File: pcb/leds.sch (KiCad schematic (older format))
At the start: 15 parts, among them J11 +5V, J12 DATA, J13 GND

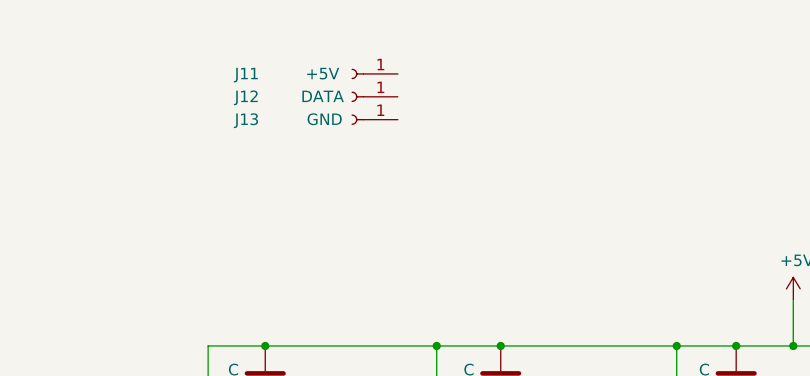
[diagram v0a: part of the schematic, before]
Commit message: update
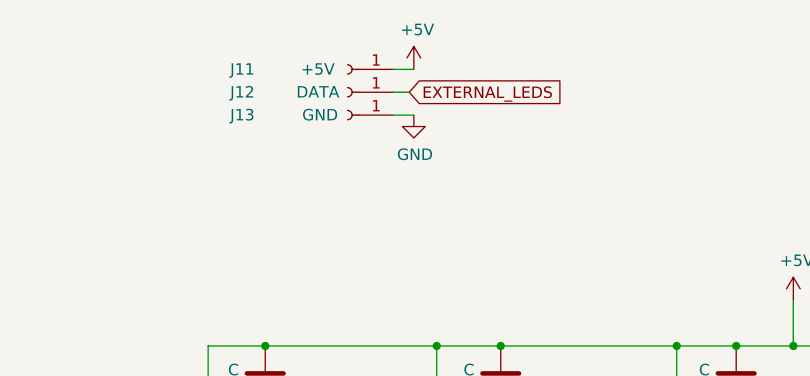
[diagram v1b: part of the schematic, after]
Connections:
- net labels added: EXTERNAL_LEDS
- wire segments 34 -> 37
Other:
- moved on the sheet: J11, J12, J13
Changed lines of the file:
@@
 L Connector:Conn_01x01_Female J?
 U 1 1 61EFE4C5
-P 4670 2340
+P 4650 2320
 AR Path="/61EFE4C5" Ref="J?"  Part="1"
 AR Path="/61B99CE8/61EFE4C5" Ref="J?"  Part="1"
 AR Path="/61B54BD1/61EFE4C5" Ref="J11"  Part="1"
-F 0 "J11" H 5130 2340 50  0000 C CNN
-F 1 "+5V" H 4800 2340 50  0000 C CNN
-F 2 "TestPoint:TestPoint_Pad_D2.0mm" H 4670 2340 50  0001 C CNN
-F 3 "~" H 4670 2340 50  0001 C CNN
-	1    4670 2340
+F 0 "J11" H 5110 2320 50  0000 C CNN
+F 1 "+5V" H 4780 2320 50  0000 C CNN
+F 2 "TestPoint:TestPoint_Pad_D2.0mm" H 4650 2320 50  0001 C CNN
+F 3 "~" H 4650 2320 50  0001 C CNN
+	1    4650 2320
 	-1   0    0    1
 $EndComp
@@
 L Connector:Conn_01x01_Female J?
 U 1 1 61EFE4CB
-P 4670 2440
+P 4650 2420
 AR Path="/61EFE4CB" Ref="J?"  Part="1"
 AR Path="/61B99CE8/61EFE4CB" Ref="J?"  Part="1"
 AR Path="/61B54BD1/61EFE4CB" Ref="J12"  Part="1"
-F 0 "J12" H 5130 2440 50  0000 C CNN
-F 1 "DATA" H 4800 2440 50  0000 C CNN
-F 2 "TestPoint:TestPoint_Pad_D2.0mm" H 4670 2440 50  0001 C CNN
-F 3 "~" H 4670 2440 50  0001 C CNN
-	1    4670 2440
+F 0 "J12" H 5110 2420 50  0000 C CNN
+F 1 "DATA" H 4780 2420 50  0000 C CNN
+F 2 "TestPoint:TestPoint_Pad_D2.0mm" H 4650 2420 50  0001 C CNN
+F 3 "~" H 4650 2420 50  0001 C CNN
+	1    4650 2420
 	-1   0    0    1
 $EndComp
@@
 L Connector:Conn_01x01_Female J?
 U 1 1 61EFE4D1
-P 4670 2540
+P 4650 2520
 AR Path="/61EFE4D1" Ref="J?"  Part="1"
 AR Path="/61B99CE8/61EFE4D1" Ref="J?"  Part="1"
 AR Path="/61B54BD1/61EFE4D1" Ref="J13"  Part="1"
-F 0 "J13" H 5130 2540 50  0000 C CNN
-F 1 "GND" H 4790 2540 50  0000 C CNN
-F 2 "TestPoint:TestPoint_Pad_D2.0mm" H 4670 2540 50  0001 C CNN
-F 3 "~" H 4670 2540 50  0001 C CNN
-	1    4670 2540
+F 0 "J13" H 5110 2520 50  0000 C CNN
+F 1 "GND" H 4770 2520 50  0000 C CNN
+F 2 "TestPoint:TestPoint_Pad_D2.0mm" H 4650 2520 50  0001 C CNN
+F 3 "~" H 4650 2520 50  0001 C CNN
+	1    4650 2520
 	-1   0    0    1
 $EndComp
+Text GLabel 4920 2420 2    50   Input ~ 0
+EXTERNAL_LEDS
+Wire Wire Line
+	4850 2420 4920 2420
+$Comp
+L power:+5V #PWR?
+U 1 1 6250EA9C
+P 4940 2320
+AR Path="/6250EA9C" Ref="#PWR?"  Part="1"
+AR Path="/61B54BD1/6250EA9C" Ref="#PWR?"  Part="1"
+F 0 "#PWR?" H 4940 2170 50  0001 C CNN
+F 1 "+5V" H 4955 2493 50  0000 C CNN
+F 2 "" H 4940 2320 50  0001 C CNN
+F 3 "" H 4940 2320 50  0001 C CNN
+	1    4940 2320
+	1    0    0    -1
+$EndComp
+$Comp
+L power:GND #PWR?
+U 1 1 6250F11C
+P 4940 2520
+AR Path="/6250F11C" Ref="#PWR?"  Part="1"
+AR Path="/61B54BD1/6250F11C" Ref="#PWR?"  Part="1"
+F 0 "#PWR?" H 4940 2270 50  0001 C CNN
+F 1 "GND" H 4945 2347 50  0000 C CNN
+F 2 "" H 4940 2520 50  0001 C CNN
+F 3 "" H 4940 2520 50  0001 C CNN
+	1    4940 2520
+	1    0    0    -1
+$EndComp
+Wire Wire Line
+	4850 2320 4940 2320
+Wire Wire Line
+	4850 2520 4940 2520
 $EndSCHEMATC
